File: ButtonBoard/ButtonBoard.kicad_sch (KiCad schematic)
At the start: 18 parts, among them J1 Conn_01x08_Socket, J2 Conn_01x08_Socket, J3 START, J4 PAUSE, J5 RESET, J6 TIME_SEL, J7 BUZZER, J8 Conn_01x06_Pin, SW1 START, SW2 PAUSE, SW3 RESET, SW4 TIME_SEL, SW5 BUZZER, U1 WEMOS_D1_mini

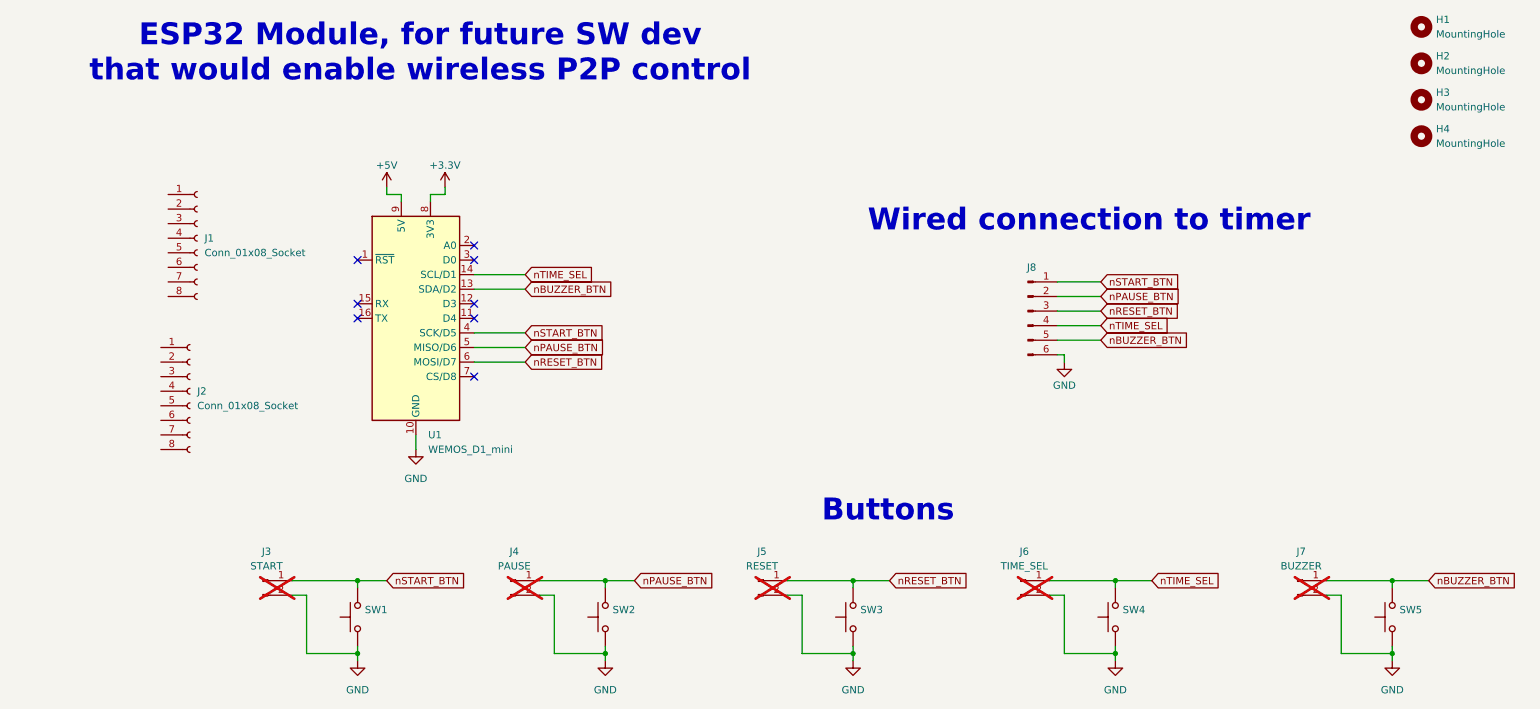
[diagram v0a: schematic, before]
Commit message: finish controller board and prod files
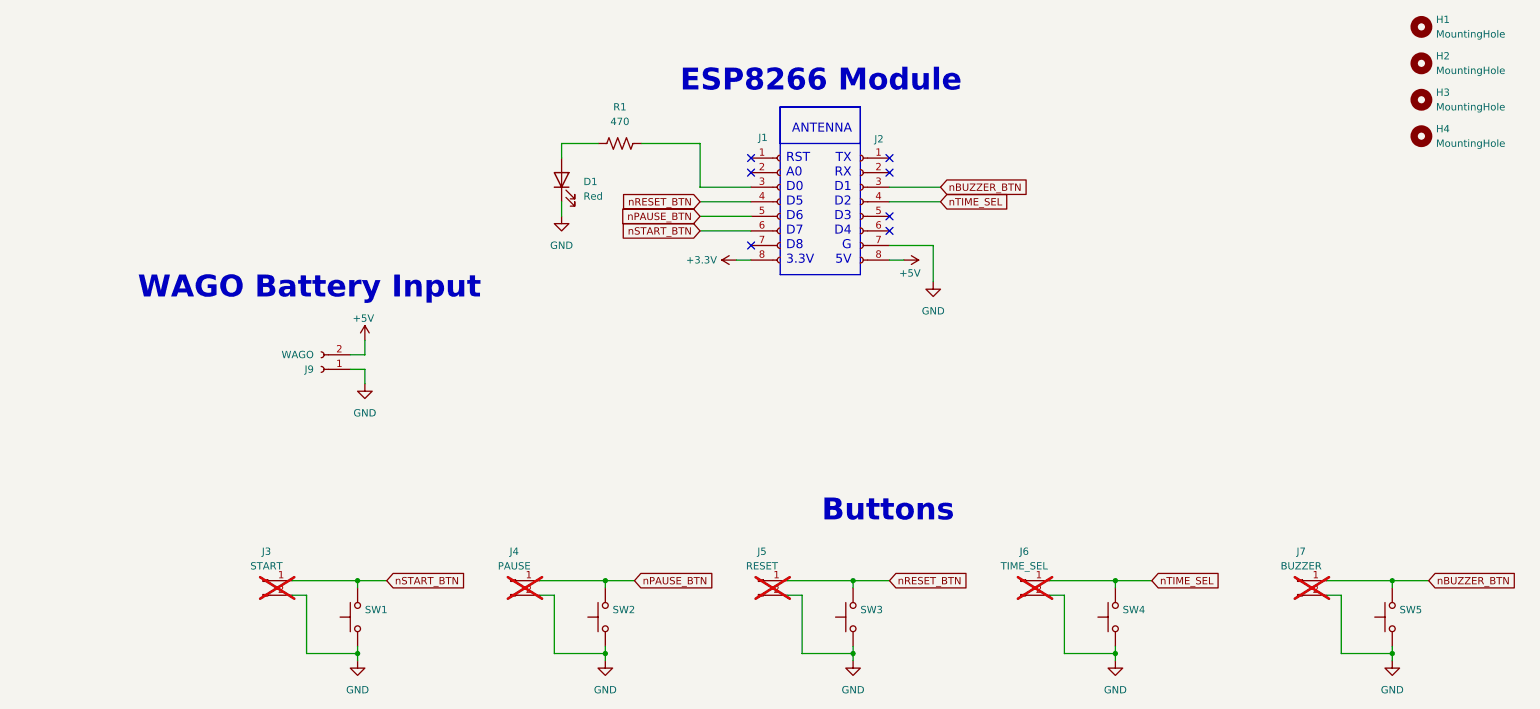
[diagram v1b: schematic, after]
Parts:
- removed J8: Conn_01x06_Pin, Connector_JST:JST_EH_S6B-EH_1x06_P2.50mm_Horizontal, symbol Connector:Conn_01x06_Pin
- removed U1: WEMOS_D1_mini, RF_Module:WEMOS_D1_mini_light, symbol RF_Module:WEMOS_D1_mini
- added D1: Red, LED_SMD:LED_0603_1608Metric, symbol Device:LED
- added J9: WAGO, WAGO_2060-452_998-404:2060-452_998-404, symbol Connector:Conn_01x02_Socket
- added R1: 470, Resistor_SMD:R_0603_1608Metric, symbol Device:R_US
- J1, J2: footprint Connector_PinHeader_2.54mm:PinHeader_1x08_P2.54mm_Vertical -> Connector_PinSocket_2.54mm:PinSocket_1x08_P2.54mm_Vertical
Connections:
- net +3.3V: now also J1.8 (Pin_8)
- net +5V: now also J2.8 (Pin_8), J9.2 (Pin_2)
- net GND: now also J2.7 (Pin_7), D1.1 (K), J9.1 (Pin_1)
- net nBUZZER_BTN: now also J2.3 (Pin_3)
- net nPAUSE_BTN: now also J1.5 (Pin_5)
- net nRESET_BTN: now also J1.4 (Pin_4)
- net nSTART_BTN: now also J1.6 (Pin_6)
- net nTIME_SEL: now also J2.4 (Pin_4)
- net at J1.3 (Pin_3): now also R1.2
- new net: D1.2 (A), R1.1
- no-connect marks 8 -> 7
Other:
- note added: "ANTENNA"
- note added: "ESP8266 Module"
- note added: "RST A0 D0 D5 D6 D7 D8 3.3V"
- note added: "TX RX D1 D2 D3 D4 G 5V"
- note added: "WAGO Battery Input"
- note removed: "ESP32 Module, for future SW dev that would enable wireless P2P control"
- note removed: "Wired connection to timer"
- moved on the sheet: J1, J2
